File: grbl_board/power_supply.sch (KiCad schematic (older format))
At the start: 26 parts, among them J5 32VDC, U3 LT1962-5, U4 BD9G341EFJ

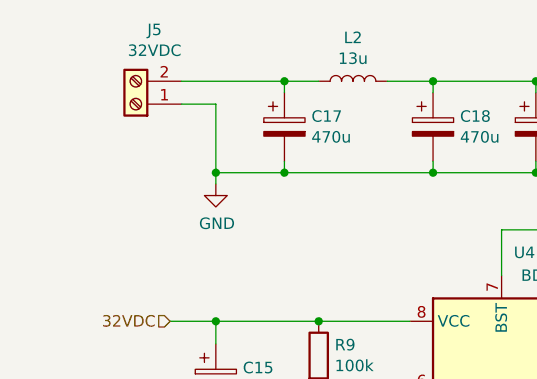
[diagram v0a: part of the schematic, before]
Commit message: routing done
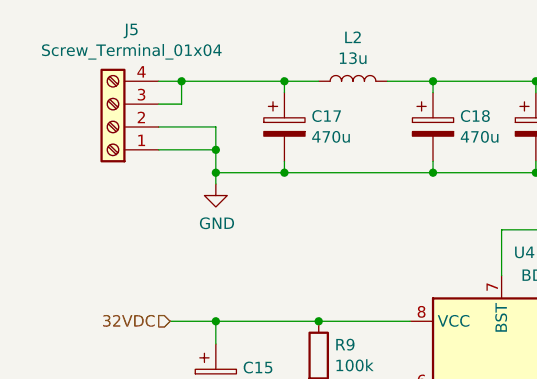
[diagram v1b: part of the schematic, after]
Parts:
- removed J5: 32VDC, Connector_Phoenix_MC:PhoenixContact_MC_1,5_2-G-3.81_1x02_P3.81mm_Horizontal, symbol Connector:Screw_Terminal_01x02
- added J5: Screw_Terminal_01x04, Connector_Phoenix_MC:PhoenixContact_MC_1,5_4-G-3.81_1x04_P3.81mm_Horizontal, symbol Connector:Screw_Terminal_01x04
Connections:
- net GND: now also J5.1 (Pin_1), J5.2 (Pin_2)
- net at C17.1, L2.1: now also J5.3 (Pin_3), J5.4 (Pin_4)
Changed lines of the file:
@@
-$EndComp
-$Comp
-L Connector:Screw_Terminal_01x02 J5
-U 1 1 617A7AB6
-P 3600 1850
-F 0 "J5" H 3518 1525 50  0000 C CNN
-F 1 "32VDC" H 3518 1616 50  0000 C CNN
-F 2 "Connector_Phoenix_MC:PhoenixContact_MC_1,5_2-G-3.81_1x02_P3.81mm_Horizontal" H 3600 1850 50  0001 C CNN
-F 3 "https://www.on-shore.com/wp-content/uploads/OSTOQXX3251.pdf" H 3600 1850 50  0001 C CNN
-F 4 "ED2808-ND" H 3600 1850 50  0001 C CNN "Digikey Part No."
-	1    3600 1850
-	-1   0    0    1
 $EndComp
 $Comp
@@
 $EndComp
 Wire Wire Line
-	3950 1850 3800 1850
-Wire Wire Line
 	5350 2150 5350 2100
 Wire Wire Line
@@
 Text HLabel 6350 1750 2    50   Input ~ 0
 32VDC
-Wire Wire Line
-	3950 1850 3950 2150
 $Comp
 L Device:L L2
@@
 Wire Wire Line
 	3950 2150 4250 2150
-Connection ~ 3950 2150
 Wire Wire Line
 	3950 2150 3950 2200
@@
 	1    0    0    -1
 $EndComp
+$Comp
+L Connector:Screw_Terminal_01x04 J5
+U 1 1 61EF7F56
+P 3500 1950
+F 0 "J5" H 3418 1525 50  0000 C CNN
+F 1 "Screw_Terminal_01x04" H 3418 1616 50  0000 C CNN
+F 2 "Connector_Phoenix_MC:PhoenixContact_MC_1,5_4-G-3.81_1x04_P3.81mm_Horizontal" H 3500 1950 50  0001 C CNN
+F 3 "https://www.on-shore.com/wp-content/uploads/OSTOQXX3251.pdf" H 3500 1950 50  0001 C CNN
+F 4 "ED2810-ND" H 3500 1950 50  0001 C CNN "Digikey Part No."
+	1    3500 1950
+	-1   0    0    1
+$EndComp
+Wire Wire Line
+	3700 1950 3950 1950
+Wire Wire Line
+	3950 1950 3950 2050
+Connection ~ 3950 2150
+Wire Wire Line
+	3950 2050 3700 2050
+Connection ~ 3950 2050
+Wire Wire Line
+	3950 2050 3950 2150
+Wire Wire Line
+	3700 1850 3800 1850
+Wire Wire Line
+	3800 1850 3800 1750
+Wire Wire Line
+	3800 1750 3700 1750
+Connection ~ 3800 1750
 $EndSCHEMATC

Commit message: updated README
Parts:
- C22: footprint Capacitor_SMD:C_1206_3216Metric_Pad1.33x1.80mm_HandSolder -> Capacitor_SMD:C_0603_1608Metric_Pad1.08x0.95mm_HandSolder; Digikey Part No. CL31F105ZBFNNNE -> 1276-1009-1-ND
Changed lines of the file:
@@
 F 0 "C22" H 6215 5046 50  0000 L CNN
 F 1 "10n" H 6215 4955 50  0000 L CNN
-F 2 "Capacitor_SMD:C_1206_3216Metric_Pad1.33x1.80mm_HandSolder" H 6138 4850 50  0001 C CNN
+F 2 "Capacitor_SMD:C_0603_1608Metric_Pad1.08x0.95mm_HandSolder" H 6138 4850 50  0001 C CNN
 F 3 "http://www.samsungsem.com/kr/support/product-search/mlcc/CL31F105ZBFNNNE.jsp" H 6100 5000 50  0001 C CNN
-F 4 "CL31F105ZBFNNNE" H 6100 5000 50  0001 C CNN "Digikey Part No."
+F 4 "1276-1009-1-ND" H 6100 5000 50  0001 C CNN "Digikey Part No."
 	1    6100 5000
 	1    0    0    -1
